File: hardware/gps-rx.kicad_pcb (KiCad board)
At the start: 4 copper layers, 22 x 22 mm, 51 parts, among them J1 Conn_01x04_Pin, J2 Conn_Coaxial_Small, U1 ICE40UP5K-SG48I, U2 MAX2769C, U3 PAM2305CGF120, U4 W25Q16JVUXIQ, Y1 1XXB16368MBA

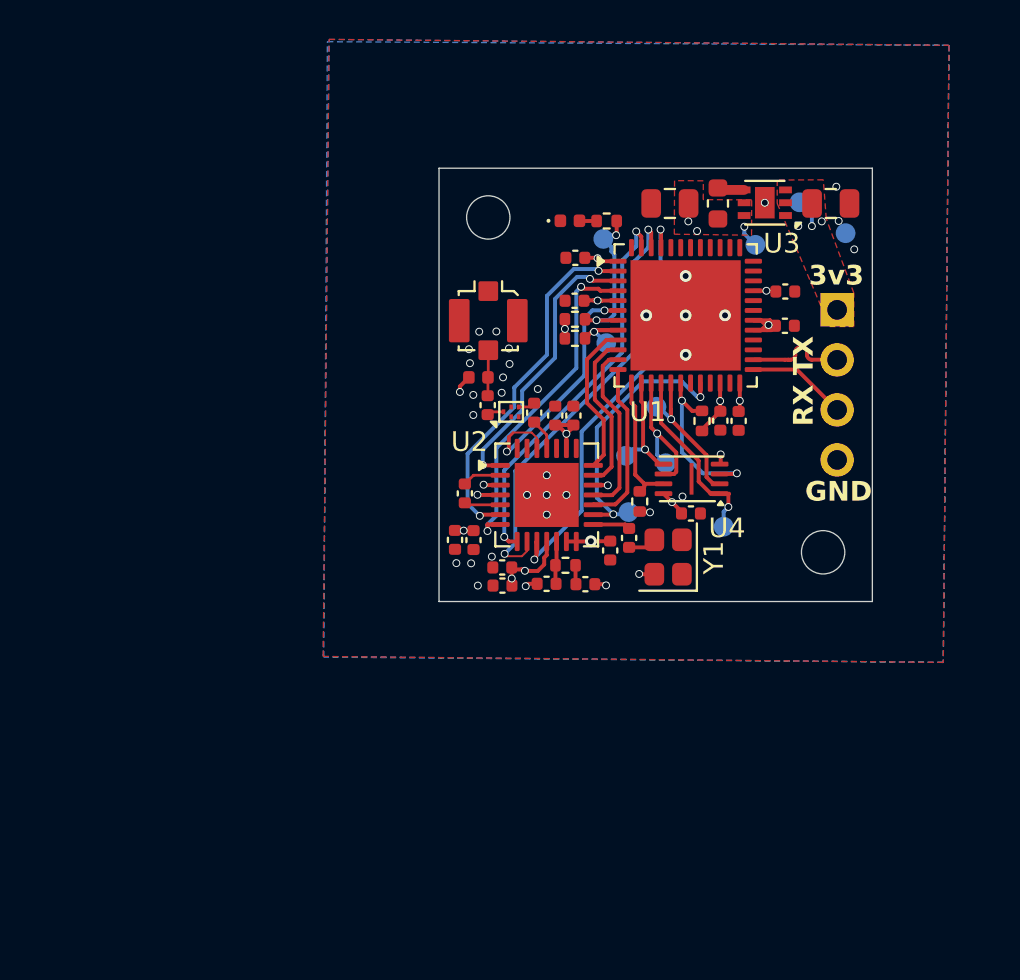
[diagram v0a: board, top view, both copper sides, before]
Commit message: new PCB design
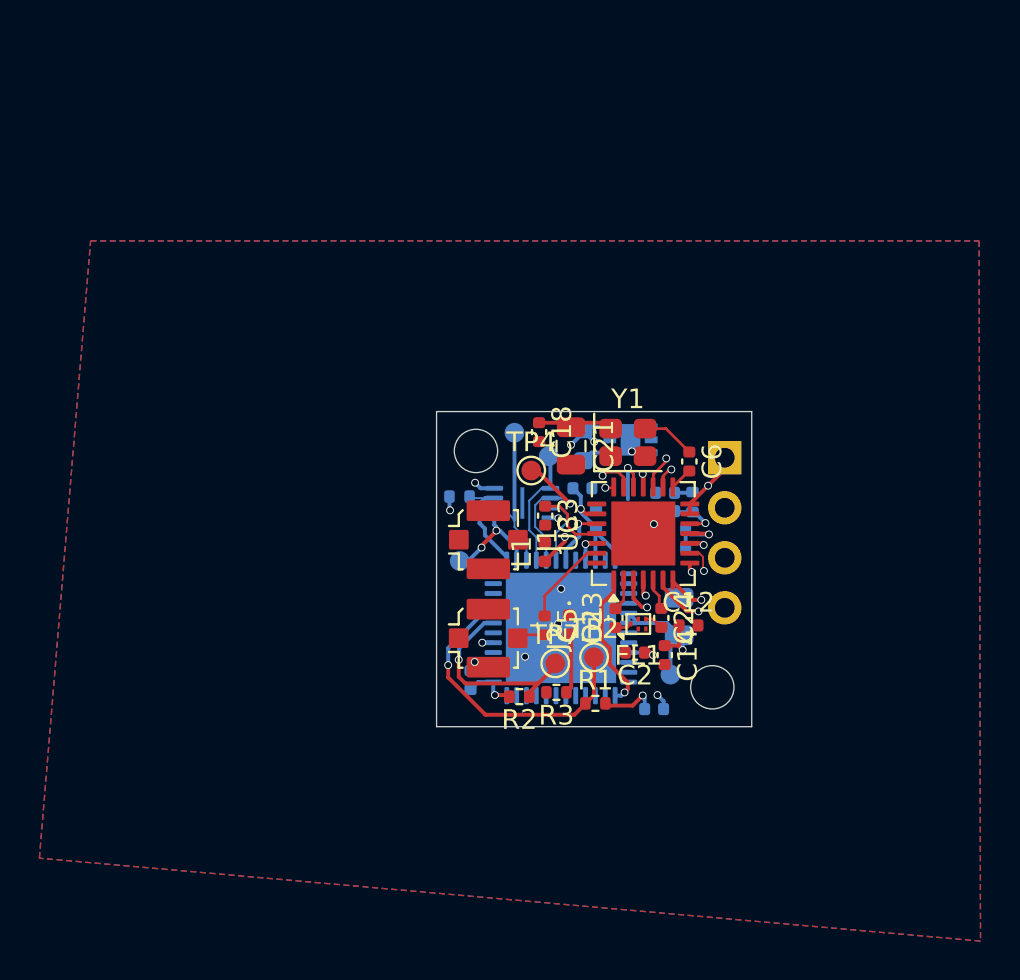
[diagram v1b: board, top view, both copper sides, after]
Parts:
- removed C1, C10, C16, C17: 100n, Capacitor_SMD:C_0402_1005Metric
- removed C7: 470p, Capacitor_SMD:C_0402_1005Metric
- removed R5: 10k, Resistor_SMD:R_0402_1005Metric
- removed TP1, TP8, TP9: TestPoint, TestPoint:TestPoint_Pad_D1.0mm
- removed U1: ICE40UP5K-SG48I, Package_DFN_QFN:QFN-48-1EP_7x7mm_P0.5mm_EP5.6x5.6mm
- added C23: 470p, Capacitor_SMD:C_0402_1005Metric, F.Cu at (176.0, 98.8)
- added C24: 470p, Capacitor_SMD:C_0402_1005Metric, F.Cu at (178.3, 98.8)
- added J3: Conn_01x04_Pin, Connector_PinHeader_2.54mm:PinHeader_1x04_P2.54mm_Vertical, B.Cu at (181.5, 90.7)
- added U5: W25Q16JVUXIQ, Package_SON:Winbond_USON-8-1EP_3x2mm_P0.5mm_EP0.2x1.6mm, B.Cu at (171.2, 93.0)
- C11, C13, C15, C19, C20, C22, C4, C8, C9, L2, R4, R6: moved to B.Cu
- H2, TP2, TP4, TP7: moved to F.Cu
- J1: value Conn_01x04_Pin -> Conn_Coaxial_Small; footprint Connector_PinHeader_2.54mm:PinHeader_1x04_P2.54mm_Vertical -> Connector_Coaxial:U.FL_Molex_MCRF_73412-0110_Vertical; moved to F.Cu
- U2: value MAX2769C -> ICE40UP5K-SG48I; footprint Package_DFN_QFN:TQFN-28-1EP_5x5mm_P0.5mm_EP3.25x3.25mm -> Package_DFN_QFN:QFN-48-1EP_7x7mm_P0.5mm_EP5.6x5.6mm; moved to B.Cu
- U3: value PAM2305CGF120 -> MAX2769C; footprint Package_DFN_QFN:DFN-6-1EP_2x2mm_P0.65mm_EP1x1.6mm -> Package_DFN_QFN:TQFN-28-1EP_5x5mm_P0.5mm_EP3.25x3.25mm
- U4: value W25Q16JVUXIQ -> PAM2305CGF120; footprint Package_SON:Winbond_USON-8-1EP_3x2mm_P0.5mm_EP0.2x1.6mm -> Package_DFN_QFN:DFN-6-1EP_2x2mm_P0.65mm_EP1x1.6mm; moved to B.Cu
- moved R3 24.1 mm to (173.0, 102.6), turned to 180 degrees
- moved TP10 22.2 mm to (178.8, 101.7)
- moved C8 22.1 mm to (168.6, 102.0), turned to 90 degrees
- moved TP7 21.7 mm to (172.9, 101.1)
- moved J1 21.2 mm to (169.5, 94.9), turned to 90 degrees
- moved C22 21.0 mm to (179.2, 98.8), turned to 90 degrees
- moved D1 20.5 mm to (173.6, 99.2), turned to -90 degrees
- moved C2 19.9 mm to (176.9, 100.6), turned to 180 degrees
- moved R2 19.4 mm to (171.1, 102.8)
- moved R1 18.6 mm to (174.9, 103.2), turned to 0 degrees
- moved C21 18.0 mm to (173.7, 90.1), turned to -90 degrees
- moved U3 17.9 mm to (177.4, 94.5), turned to 90 degrees
- moved C14 17.8 mm to (178.5, 100.7), turned to -90 degrees
- moved C12 17.5 mm to (179.7, 99.2), turned to 0 degrees
- moved J2 16.1 mm to (169.5, 99.9), turned to 90 degrees
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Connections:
- C3 pad 1: Net-(C3-Pad1) -> /ACTIVE
- C3 pad 2: Net-(J2-In) -> Net-(J1-In)
- C5 pad 1: Net-(U3-LNA2) -> /PASSIVE
- C5 pad 2: Net-(C5-Pad2) -> Net-(J2-In)
- FL1 pad 1: Net-(C3-Pad1) -> Net-(C23-Pad1)
- FL1 pad 4: Net-(C5-Pad2) -> Net-(C24-Pad2)
- J1 pad 1: +3V3 -> Net-(J1-In)
- J1 pad 2: /TX -> GND
- L1 pad 2: Net-(J2-In) -> Net-(J1-In)
- U2 pad 1: /ANTFLAG -> +3V3
- U2 pad 10: /~{CS} -> unconnected-(U2B-IOB_18a-Pad10)
- U2 pad 11: +3V3 -> unconnected-(U2B-IOB_20a-Pad11)
- U2 pad 12: Net-(U3-CPOUT) -> unconnected-(U2B-IOB_22a-Pad12)
- U2 pad 13: +3V3 -> /qSPI_~{RESET}
- U2 pad 14: +3V3 -> /qSPI_SO
- U2 pad 15: Net-(U3-XTAL) -> /qSPI_CLK
- U2 pad 16: /CLKOUT -> /qSPI_~{CS}
- U2 pad 17: /Q1 -> /qSPI_SI
- U2 pad 18: /Q0 -> /qSPI_~{WP}
- U2 pad 19: +3V3 -> /~{IDLE}
- U2 pad 2: /LNAOUT -> unconnected-(U2C-IOB_6a-Pad2)
- U2 pad 20: /I0 -> /CLKOUT
- U2 pad 21: /I1 -> /PGM
- U2 pad 22: unconnected-(U3-NC-Pad22) -> +3V3
- U2 pad 23: +3V3 -> unconnected-(U2A-IOT_37a-Pad23)
- U2 pad 24: /~{IDLE} -> +3V3
- U2 pad 25: Net-(U3-LNA2) -> unconnected-(U2A-IOT_36b-Pad25)
- U2 pad 26: /PGM -> unconnected-(U2A-IOT_39a-Pad26)
- U2 pad 29: GND -> +1V2
- U2 pad 3: /ANTIBIAS -> unconnected-(U2C-IOB_9b-Pad3)
- U2 pad 4: +3V3 -> unconnected-(U2C-IOB_8a-Pad4)
- U2 pad 5: /MIXIN -> +1V2
- U2 pad 6: /LD -> unconnected-(U2B-IOB_13b-Pad6)
- U2 pad 7: /~{SHDN} -> /CDONE
- U2 pad 8: /SDATA -> /~{CRESET}
- U2 pad 9: /SCLK -> unconnected-(U2B-IOB_16a-Pad9)
- U3 pad 1: unconnected-(U4-NC-Pad1) -> /ANTFLAG
- U3 pad 2: +3V3 -> /LNAOUT
- U3 pad 3: +3V3 -> /ANTIBIAS
- U3 pad 4: Net-(U4-SW) -> +3V3
- U3 pad 5: GND -> /MIXIN
- U3 pad 6: +1V2 -> /LD
- U3 pad 7: GND -> /~{SHDN}
- U4 pad 1: /qSPI_~{CS} -> unconnected-(U4-NC-Pad1)
- U4 pad 2: /qSPI_SI -> +3V3
- U4 pad 3: /qSPI_~{WP} -> +3V3
- U4 pad 4: GND -> Net-(U4-SW)
- U4 pad 5: /qSPI_SO -> GND
- U4 pad 6: /qSPI_CLK -> +1V2
- U4 pad 7: /qSPI_~{RESET} -> GND
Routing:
- net /~{CS}: track 21.9 -> 0.74 mm, vias 2 -> 1
- net /SCLK: track 22.2 -> 1.49 mm, vias 2 -> 1
- net /SDATA: track 20.0 -> 0.49 mm, vias 2 -> 1
- net /LD: track 18.4 -> 2.67 mm, vias 2 -> 1
- net /~{SHDN}: track 17.4 -> 1.91 mm, vias 2 -> 1
- net /CLKOUT: track 13.9 -> 1.11 mm, vias 2 -> 1
- net /PGM: track 13.3 -> 1.41 mm, vias 2 -> 1
- net /~{CRESET}: track 3.98 -> 15.0 mm
- net /Q0: track 8.93 -> 0.68 mm, vias 0 -> 1
- net /I1: track 7.93 -> 0.45 mm, vias 0 -> 1
- net /ANTFLAG: track 14.6 -> 7.13 mm, vias 2 -> 1
- net +1V2: track 7.56 -> 14.6 mm, vias 5 -> 4
- net /Q1: track 8.43 -> 1.86 mm, vias 0 -> 1
- net /I0: track 8.19 -> 1.74 mm, vias 0 -> 1
- net +3V3: track 24.3 -> 30.1 mm, vias 18 -> 10
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- removed copper zone on F.Cu, net +1V2
- removed copper zone on In2.Cu, net +1V2
- removed copper zone on B.Cu, net +3V3
- removed copper zone on F.Cu, net +3V3
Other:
- board size 22 x 22 mm -> 16 x 16 mm
- board text removed: "3v3"
- board text removed: "GND"
- board text removed: "RX TX"

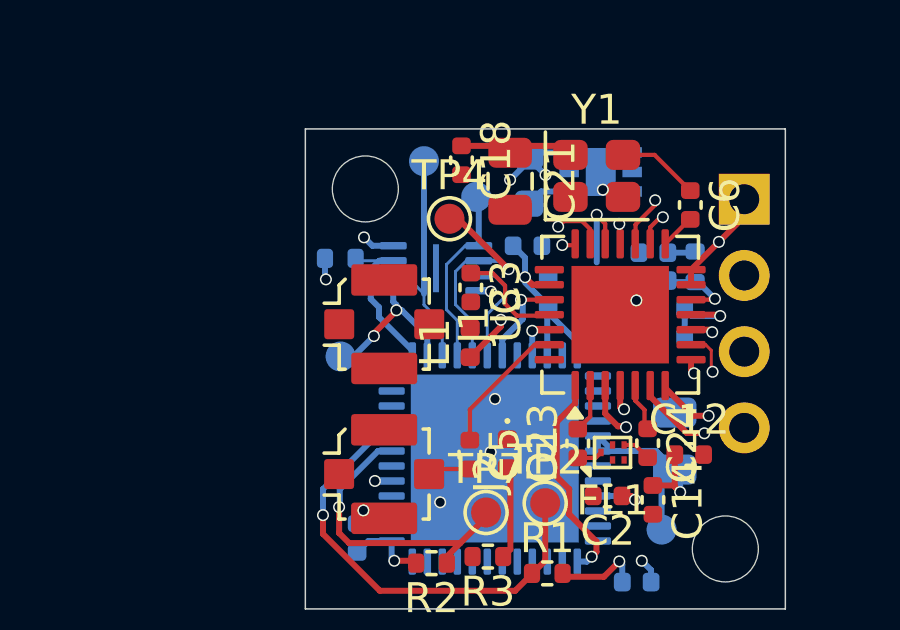
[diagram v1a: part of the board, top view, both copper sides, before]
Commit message: working
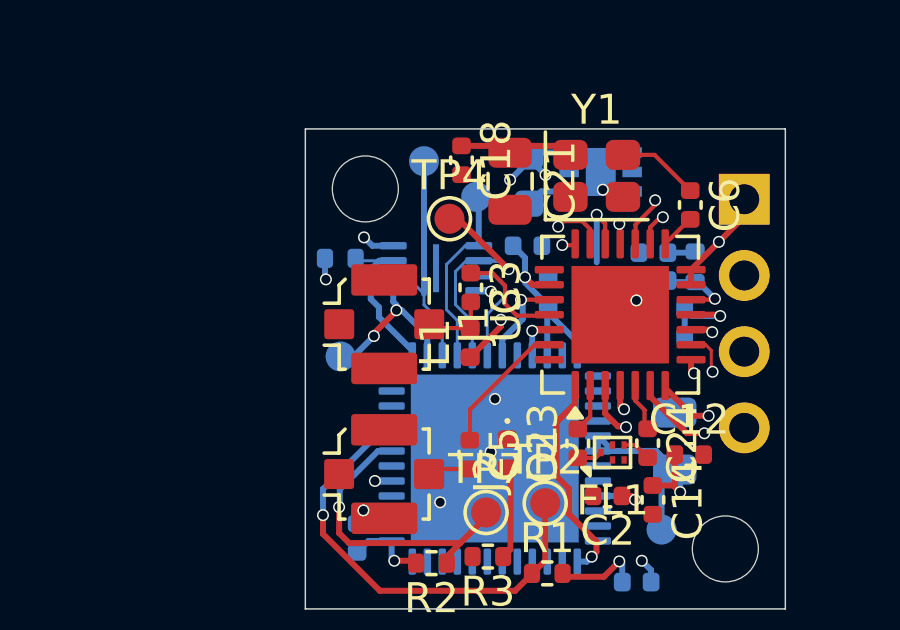
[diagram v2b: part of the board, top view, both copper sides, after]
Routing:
- net Net-(J1-In): track 0.00 -> 2.30 mm

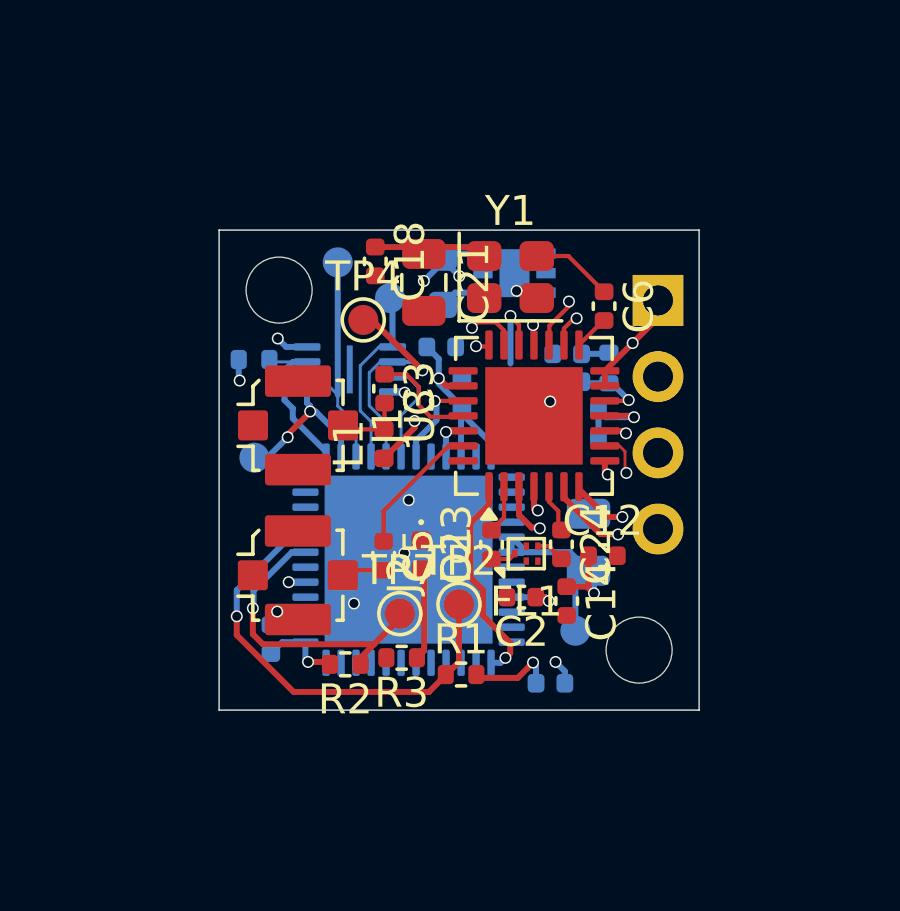
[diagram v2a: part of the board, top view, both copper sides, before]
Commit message: PCB completed
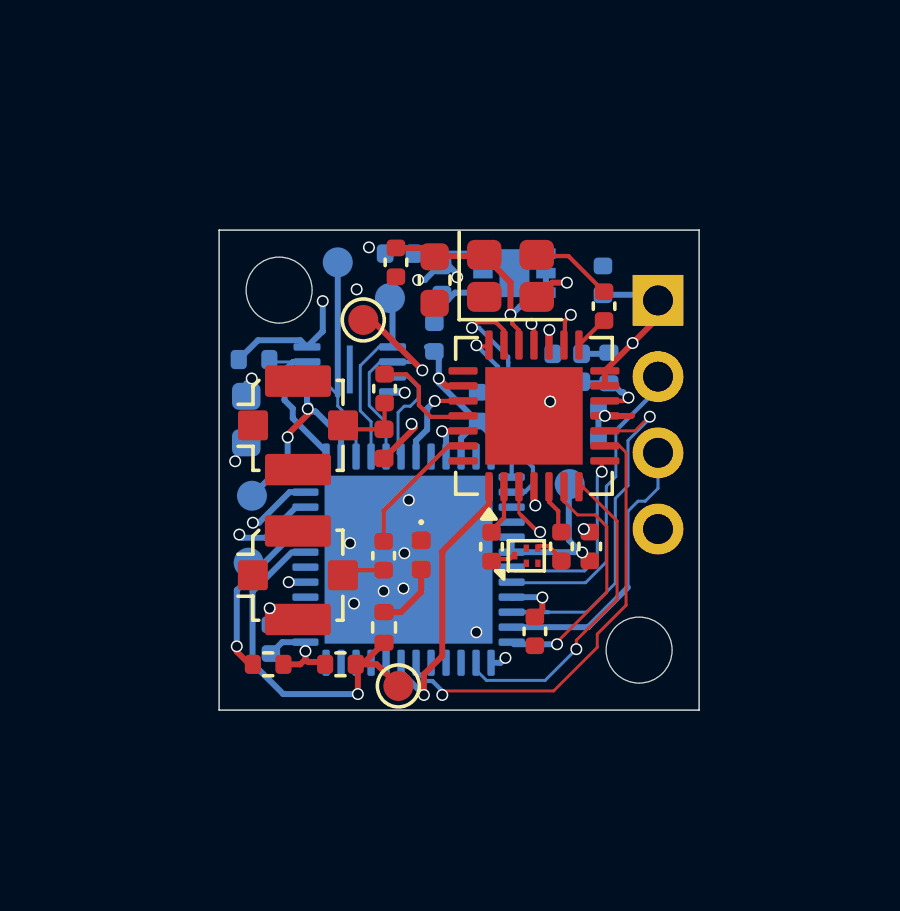
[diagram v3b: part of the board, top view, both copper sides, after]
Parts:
- C14, TP2: moved to B.Cu
- C21, C22: footprint Capacitor_SMD:C_0805_2012Metric -> Capacitor_SMD:C_0603_1608Metric
- L2: value L -> 2.2u; footprint Inductor_SMD:L_0603_1608Metric -> Inductor_SMD:L_0402_1005Metric
- R3: value 220R -> 1k
- moved C15 13.5 mm to (179.7, 90.0), turned to 90 degrees
- moved C14 12.8 mm to (172.9, 89.1), turned to 180 degrees
- moved C22 12.1 mm to (167.8, 94.7), turned to -90 degrees
- moved TP2 7.15 mm to (167.9, 99.4), turned to 180 degrees
- moved R1 6.44 mm to (168.5, 102.8)
- moved TP10 4.89 mm to (178.6, 96.8)
- moved TP7 2.41 mm to (172.8, 103.5)
- moved TP3 1.27 mm to (168.0, 97.2)
- moved C2 1.23 mm to (177.4, 101.7), turned to -90 degrees
- moved R3 1.17 mm to (172.4, 101.6), turned to -90 degrees
- moved C4 0.72 mm to (175.5, 94.2)
- moved C18 0.69 mm to (172.8, 89.4)
- moved C12 0.54 mm to (179.2, 98.9), turned to 90 degrees
- moved C9 0.40 mm to (174.1, 91.9), turned to 90 degrees
- moved C21 0.37 mm to (174.1, 90.0)
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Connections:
- U2 pad 10: unconnected-(U2B-IOB_18a-Pad10) -> /Q1
- U2 pad 11: unconnected-(U2B-IOB_20a-Pad11) -> /Q0
- U2 pad 20: /CLKOUT -> unconnected-(U2B-IOB_25b_G3-Pad20)
- U2 pad 25: unconnected-(U2A-IOT_36b-Pad25) -> /I1
- U2 pad 26: unconnected-(U2A-IOT_39a-Pad26) -> /I0
- U2 pad 31: unconnected-(U2A-IOT_42b-Pad31) -> /SDATA
- U2 pad 32: unconnected-(U2A-IOT_43a-Pad32) -> /TX
- U2 pad 34: unconnected-(U2A-IOT_44b-Pad34) -> /~{CS}
- U2 pad 35: unconnected-(U2A-IOT_46b_G0-Pad35) -> /RX
- U2 pad 36: unconnected-(U2A-IOT_48b-Pad36) -> /LD
- U2 pad 37: /ANTFLAG -> /CLKOUT
- U2 pad 38: unconnected-(U2A-IOT_50b-Pad38) -> /~{SHDN}
- U2 pad 42: unconnected-(U2A-IOT_51a-Pad42) -> /SCLK
- U2 pad 43: unconnected-(U2A-IOT_49a-Pad43) -> /ANTFLAG
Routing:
- net /Q0: track 0.68 -> 29.4 mm, vias 1 -> 2
- net /Q1: track 1.86 -> 30.6 mm, vias 1 -> 2
- net /CLKOUT: track 1.11 -> 17.3 mm, vias 1 -> 2
- net /SCLK: track 1.49 -> 14.9 mm
- net /~{CS}: track 0.74 -> 11.6 mm
- net /TX: track 0.00 -> 10.3 mm
- net +3V3: track 30.1 -> 40.0 mm, vias 10 -> 8
- net /RX: track 0.00 -> 9.69 mm
- net /~{CRESET}: track 15.0 -> 5.78 mm
- net /~{SHDN}: track 1.91 -> 10.5 mm
- net /I0: track 1.74 -> 8.75 mm
- net /LD: track 2.67 -> 8.68 mm
- net /SDATA: track 0.49 -> 6.49 mm
- net /I1: track 0.45 -> 5.34 mm
- net +1V2: track 14.6 -> 11.6 mm, vias 4 -> 5
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- added copper zone on In2.Cu, net +1V2
